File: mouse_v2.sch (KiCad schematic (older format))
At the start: 105 parts, among them J1 HC05 Header, J2 Serial Debug Header, J3 HC05_Key Jump, J4 Conn_ARM_JTAG_SWD_10, J5 SWD Header, J6 Conn_01x02_Female, J7 Conn_01x02_Female, J8 Conn_01x02_Female, J9 Conn_01x02_Female, M1 M1_Conn, M2 M2_Conn, M3 M1_Conn_Alt, M4 M2_Conn_Alt, Q0 Q_Photo_NPN, Q1 Q_Photo_NPN, Q2 Q_Photo_NPN, Q3 Q_Photo_NPN, Q4 Q_NMOS_SGD, Q5 Q_NMOS_SGD, Q6 Q_NMOS_SGD, Q7 Q_NMOS_SGD, Q8 Q_NMOS_SGD, SW1 SW, U1 YAAJ_BluePill_SWD_Breakout, U2 L293D, U3 LM1085-5.0, U4 APE8865Y5-33-HF-3

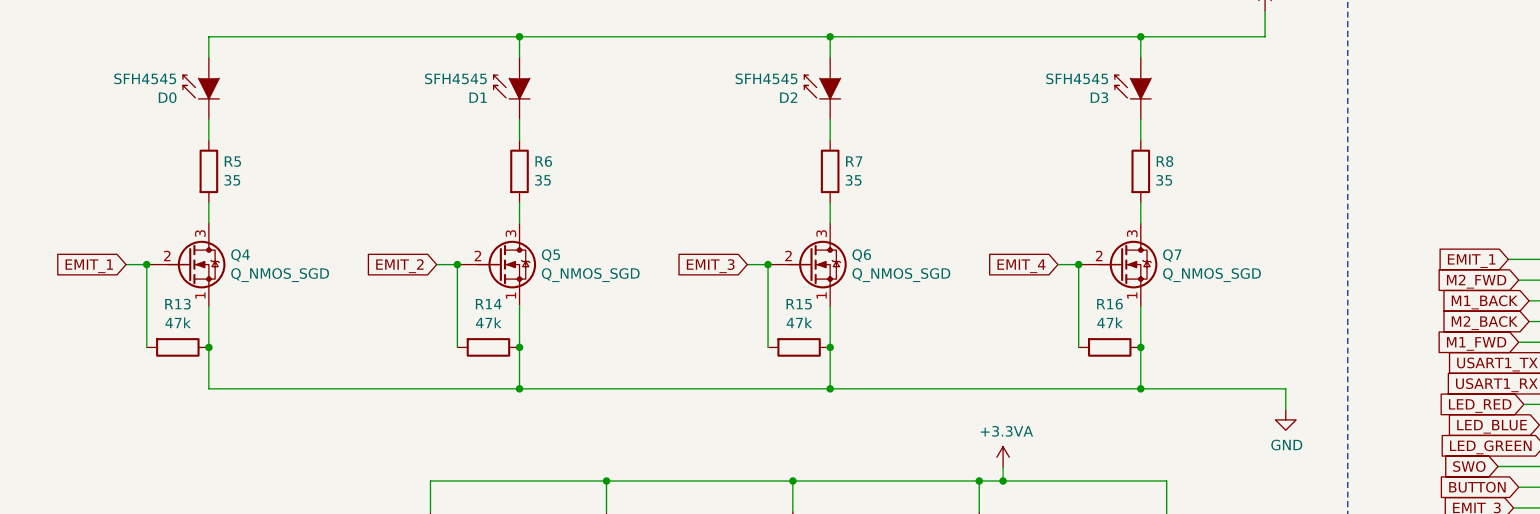
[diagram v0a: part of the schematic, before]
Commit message: tracing
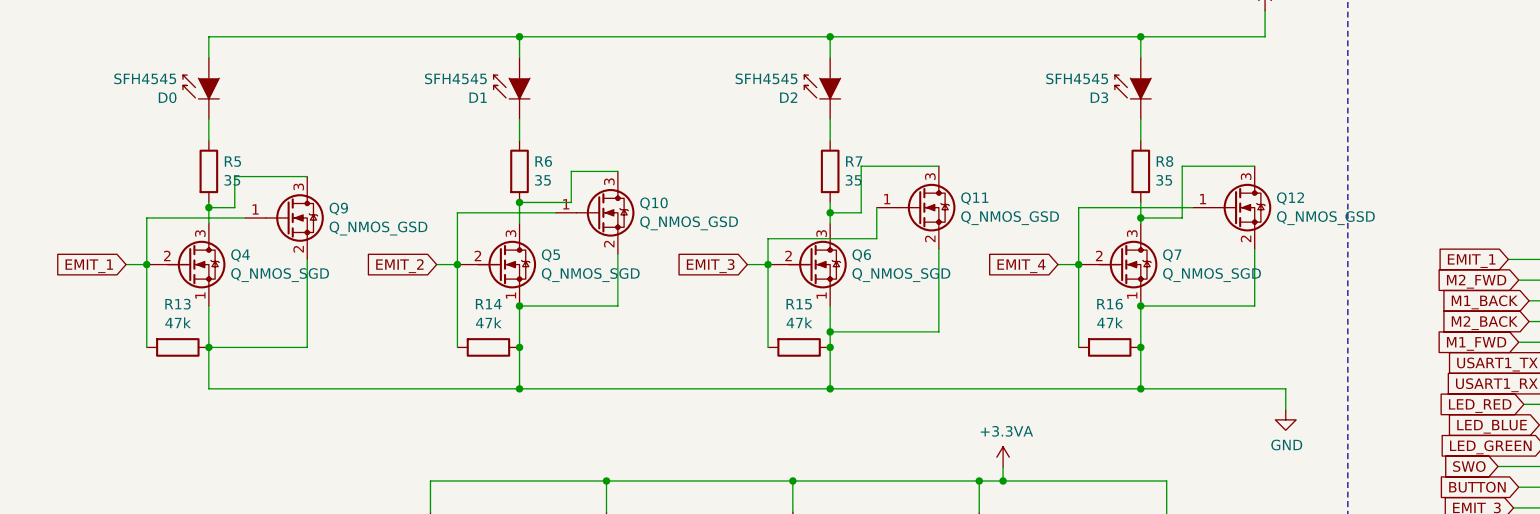
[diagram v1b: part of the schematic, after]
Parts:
- added Q10, Q11, Q12, Q9: Q_NMOS_GSD, Package_TO_SOT_SMD:SOT-23, symbol Device:Q_NMOS_GSD
- U3: footprint Package_TO_SOT_SMD:TO-263-3_TabPin2 -> custom:VREG_TO-263-3_TabPin2
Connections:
- net EMIT_1: now also Q9.1 (G)
- net EMIT_2: now also Q10.1 (G)
- net EMIT_3: now also Q11.1 (G)
- net EMIT_4: now also Q12.1 (G)
- net GND: now also Q10.2 (S), Q11.2 (S), Q12.2 (S), Q9.2 (S)
- net at Q7.3 (D), R8.2: now also Q12.3 (D)
- net at Q6.3 (D), R7.2: now also Q11.3 (D)
- net at Q4.3 (D), R5.2: now also Q9.3 (D)
- net at Q5.3 (D), R6.2: now also Q10.3 (D)
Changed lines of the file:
@@
 F 0 "U3" H 4225 6917 50  0000 C CNN
 F 1 "LM1085-5.0" H 4225 6826 50  0000 C CNN
-F 2 "Package_TO_SOT_SMD:TO-263-3_TabPin2" H 4225 6925 50  0001 C CIN
+F 2 "custom:VREG_TO-263-3_TabPin2" H 4225 6925 50  0001 C CIN
 F 3 "http://www.ti.com/lit/ds/symlink/lm1084.pdf" H 4225 6675 50  0001 C CNN
 	1    4225 6675
@@
 	900  2000 1000 2000
 Wire Wire Line
-	1300 1700 1300 1800
+	1300 1700 1300 1725
 Wire Wire Line
 	1300 1300 1300 1400
@@
 	3900 2000 4000 2000
 Wire Wire Line
-	4300 1700 4300 1800
+	4300 1700 4300 1750
 Wire Wire Line
 	4300 1300 4300 1400
@@
 Wire Wire Line
 	4000 2000 4000 2400
-Wire Wire Line
-	4300 2200 4300 2400
 $Comp
 L mouse_v2-rescue:IRL81A-LED D2
@@
 Wire Wire Line
 	5400 2000 5500 2000
-Wire Wire Line
-	5800 1700 5800 1800
 Wire Wire Line
 	5800 1300 5800 1400
@@
 	5135 3045 5925 3045
 $Comp
-L power:GND #PWR?
+L power:GND #PWR0107
 U 1 1 63794FA2
 P 13300 3375
-F 0 "#PWR?" H 13300 3125 50  0001 C CNN
+F 0 "#PWR0107" H 13300 3125 50  0001 C CNN
 F 1 "GND" H 13305 3202 50  0000 C CNN
 F 2 "" H 13300 3375 50  0001 C CNN
@@
 	1    0    0    -1
 $EndComp
+Wire Wire Line
+	6350 1925 6350 2200
+Wire Wire Line
+	6350 2200 5800 2200
+Connection ~ 5800 2200
+Wire Wire Line
+	5500 1725 5500 2000
+Wire Wire Line
+	4825 1525 4450 1525
+Wire Wire Line
+	4450 1525 4450 1750
+Wire Wire Line
+	4450 1750 4300 1750
+Connection ~ 4300 1750
+Wire Wire Line
+	4300 1750 4300 1800
+Wire Wire Line
+	4525 1725 4525 1875
+Wire Wire Line
+	4525 1875 4000 1875
+Wire Wire Line
+	4000 1875 4000 2000
+Wire Wire Line
+	4825 1925 4825 2325
+Wire Wire Line
+	4825 2325 4300 2325
+Wire Wire Line
+	4300 2200 4300 2325
+Connection ~ 4300 2325
+Wire Wire Line
+	4300 2325 4300 2400
+Wire Wire Line
+	3275 1950 3275 2200
+Wire Wire Line
+	3275 2200 2800 2200
+Connection ~ 2800 2200
+Wire Wire Line
+	2975 1750 2500 1750
+Wire Wire Line
+	2500 1750 2500 2000
+Wire Wire Line
+	3275 1550 3050 1550
+Wire Wire Line
+	3050 1550 3050 1700
+Wire Wire Line
+	3050 1700 2800 1700
+Connection ~ 2800 1700
+Wire Wire Line
+	1775 1575 1425 1575
+Wire Wire Line
+	1425 1575 1425 1725
+Wire Wire Line
+	1425 1725 1300 1725
+Connection ~ 1300 1725
+Wire Wire Line
+	1300 1725 1300 1800
+Wire Wire Line
+	1775 1975 1775 2400
+Wire Wire Line
+	1775 2400 1300 2400
+$Comp
+L Device:Q_NMOS_GSD Q12
+U 1 1 638F1AA4
+P 6250 1725
+F 0 "Q12" H 6454 1771 50  0000 L CNN
+F 1 "Q_NMOS_GSD" H 6454 1680 50  0000 L CNN
+F 2 "Package_TO_SOT_SMD:SOT-23" H 6450 1825 50  0001 C CNN
+F 3 "~" H 6250 1725 50  0001 C CNN
+	1    6250 1725
+	1    0    0    -1
+$EndComp
+$Comp
+L Device:Q_NMOS_GSD Q11
+U 1 1 638F34B2
+P 4725 1725
+F 0 "Q11" H 4929 1771 50  0000 L CNN
+F 1 "Q_NMOS_GSD" H 4929 1680 50  0000 L CNN
+F 2 "Package_TO_SOT_SMD:SOT-23" H 4925 1825 50  0001 C CNN
+F 3 "~" H 4725 1725 50  0001 C CNN
+	1    4725 1725
+	1    0    0    -1
+$EndComp
+$Comp
+L Device:Q_NMOS_GSD Q10
+U 1 1 638F43B8
+P 3175 1750
+F 0 "Q10" H 3379 1796 50  0000 L CNN
+F 1 "Q_NMOS_GSD" H 3379 1705 50  0000 L CNN
+F 2 "Package_TO_SOT_SMD:SOT-23" H 3375 1850 50  0001 C CNN
+F 3 "~" H 3175 1750 50  0001 C CNN
+	1    3175 1750
+	1    0    0    -1
+$EndComp
+$Comp
+L Device:Q_NMOS_GSD Q9
+U 1 1 638F50C4
+P 1675 1775
+F 0 "Q9" H 1879 1821 50  0000 L CNN
+F 1 "Q_NMOS_GSD" H 1879 1730 50  0000 L CNN
+F 2 "Package_TO_SOT_SMD:SOT-23" H 1875 1875 50  0001 C CNN
+F 3 "~" H 1675 1775 50  0001 C CNN
+	1    1675 1775
+	1    0    0    -1
+$EndComp
+Wire Wire Line
+	6050 1725 5500 1725
+Wire Wire Line
+	5800 1700 5800 1775
+Wire Wire Line
+	5800 1775 6000 1775
+Wire Wire Line
+	6000 1775 6000 1525
+Wire Wire Line
+	6000 1525 6350 1525
+Connection ~ 5800 1775
+Wire Wire Line
+	5800 1775 5800 1800
+Wire Wire Line
+	1000 1775 1000 2000
+Wire Wire Line
+	1000 1775 1475 1775
 $EndSCHEMATC
